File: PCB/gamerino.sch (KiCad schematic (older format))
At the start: 47 parts, among them J1 USB_B_Micro, J2 LT2, J3 RT2, P1 JOY1, P2 JOY2, P3 ICSP, P4 AUX, SW1 HATSWITCH, SW10 OPTS, SW11 X, SW12 B, SW13 A, SW14 Y, SW2 LT1, SW3 LT2, SW4 RT1, SW5 RT2, SW6 SEL, SW7 START, SW8 BACK, SW9 HOME, U1 MIC5219-3.3YM5, U2 ATmega32U4, U3 TCA9539, X1 16MHz

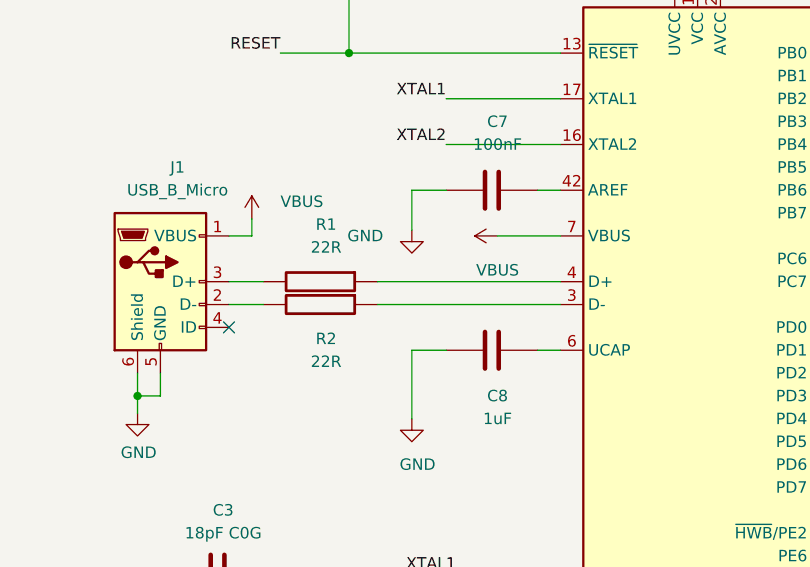
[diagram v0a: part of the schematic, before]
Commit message: Update Layout
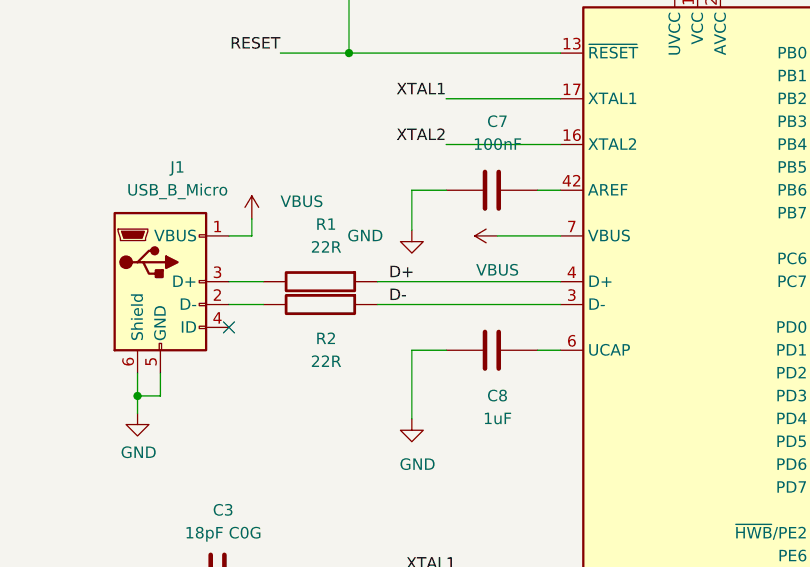
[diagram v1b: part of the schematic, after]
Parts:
- J2, J3: footprint gamerino:53398-0371 -> gamerino:Molex_PicoBlade_53047-0310_1x03_P1.25mm_Vertical
- R1, R2: footprint Resistor_SMD:R_0603_1608Metric -> Resistor_SMD:R_0402_1005Metric; MPN RT0603FRE0722RL -> (none); Manufacturer Yageo -> (none)
- SW10, SW6, SW7, SW8: footprint gamerino:TL1105-T -> gamerino:TL6210; MPN TL1105TF160Q -> TL6210AF200GQ
- SW9: footprint gamerino:TL1220 -> gamerino:TL3265; MPN TL1220R3BBBNN -> TL3265GQSCLR
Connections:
- net D-: now reaches R2.1, U2.3 (D-)
- net D+: now reaches R1.1, U2.4 (D+)
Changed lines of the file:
@@
 F 0 "R1" V 4175 4575 50  0000 C CNN
 F 1 "22R" V 4275 4575 50  0000 C CNN
-F 2 "Resistor_SMD:R_0603_1608Metric" V 4355 4550 30  0001 C CNN
+F 2 "Resistor_SMD:R_0402_1005Metric" V 4355 4550 30  0001 C CNN
 F 3 "" H 4425 4550 30  0000 C CNN
-F 4 "RT0603FRE0722RL" H 4425 4550 50  0001 C CNN "MPN"
-F 5 "Yageo" H 4425 4550 50  0001 C CNN "Manufacturer"
+F 4 "" H 4425 4550 50  0001 C CNN "MPN"
+F 5 "" H 4425 4550 50  0001 C CNN "Manufacturer"
 	1    4425 4550
 	0    1    1    0
@@
 F 0 "R2" V 4575 4675 50  0000 C CNN
 F 1 "22R" V 4675 4675 50  0000 C CNN
-F 2 "Resistor_SMD:R_0603_1608Metric" V 4355 4650 30  0001 C CNN
+F 2 "Resistor_SMD:R_0402_1005Metric" V 4355 4650 30  0001 C CNN
 F 3 "" H 4425 4650 30  0000 C CNN
-F 4 "RT0603FRE0722RL" H 4425 4650 50  0001 C CNN "MPN"
-F 5 "Yageo" H 4425 4650 50  0001 C CNN "Manufacturer"
+F 4 "" H 4425 4650 50  0001 C CNN "MPN"
+F 5 "" H 4425 4650 50  0001 C CNN "Manufacturer"
 	1    4425 4650
 	0    1    1    0
@@
 F 0 "J3" H 8050 9550 50  0000 C CNN
 F 1 "RT2" H 8050 9650 50  0000 C CNN
-F 2 "gamerino:53398-0371" H 8175 9925 50  0001 C CNN
+F 2 "gamerino:Molex_PicoBlade_53047-0310_1x03_P1.25mm_Vertical" H 8175 9925 50  0001 C CNN
 F 3 "" H 8175 9925 50  0001 C CNN
 F 4 "53047-0310" H 8175 9925 50  0001 C CNN "MPN"
@@
 F 0 "J2" H 8042 7739 50  0000 C CNN
 F 1 "LT2" H 8042 7830 50  0000 C CNN
-F 2 "gamerino:53398-0371" H 8175 8075 50  0001 C CNN
+F 2 "gamerino:Molex_PicoBlade_53047-0310_1x03_P1.25mm_Vertical" H 8175 8075 50  0001 C CNN
 F 3 "" H 8175 8075 50  0001 C CNN
 F 4 "53047-0310" H 8175 8075 50  0001 C CNN "MPN"
@@
 F 0 "SW9" H 14467 3431 50  0000 C CNN
 F 1 "HOME" H 14467 3340 50  0000 C CNN
-F 2 "gamerino:TL1220" H 14450 3250 50  0001 C CNN
+F 2 "gamerino:TL3265" H 14450 3250 50  0001 C CNN
 F 3 "" H 14450 3250 50  0001 C CNN
-F 4 "TL1220R3BBBNN" H 14450 3100 50  0001 C CNN "MPN"
+F 4 "TL3265GQSCLR" H 14450 3100 50  0001 C CNN "MPN"
 F 5 "E-Switch" H 14450 3100 50  0001 C CNN "Manufacturer"
 	1    14450 3100
@@
 F 0 "SW9" V 8846 8222 50  0000 R CNN
 F 1 "HOME" V 8755 8222 50  0000 R CNN
-F 2 "gamerino:TL1220" H 8800 8850 50  0001 C CNN
+F 2 "gamerino:TL3265" H 8800 8850 50  0001 C CNN
 F 3 "" H 8800 8850 50  0001 C CNN
-F 4 "TL1220R3BBBNN" H 8800 8700 50  0001 C CNN "MPN"
+F 4 "TL3265GQSCLR" H 8800 8700 50  0001 C CNN "MPN"
 F 5 "E-Switch" H 8800 8700 50  0001 C CNN "Manufacturer"
 	2    8800 8700
@@
 F 0 "SW6" H 14467 1781 50  0000 C CNN
 F 1 "SEL" H 14467 1690 50  0000 C CNN
-F 2 "gamerino:TL1105-T" H 14450 1100 50  0001 C CNN
+F 2 "gamerino:TL6210" H 14450 1100 50  0001 C CNN
 F 3 "" H 14450 1100 50  0001 C CNN
-F 4 "TL1105TF160Q" H 14450 1450 50  0001 C CNN "MPN"
+F 4 "TL6210AF200GQ" H 14450 1450 50  0001 C CNN "MPN"
 F 5 "E-Switch" H 14450 1450 50  0001 C CNN "Manufacturer"
 	1    14450 1450
@@
 F 0 "SW7" H 14467 2306 50  0000 C CNN
 F 1 "START" H 14467 2215 50  0000 C CNN
-F 2 "gamerino:TL1105-T" H 14450 1625 50  0001 C CNN
+F 2 "gamerino:TL6210" H 14450 1625 50  0001 C CNN
 F 3 "" H 14450 1625 50  0001 C CNN
-F 4 "TL1105TF160Q" H 14450 1975 50  0001 C CNN "MPN"
+F 4 "TL6210AF200GQ" H 14450 1975 50  0001 C CNN "MPN"
 F 5 "E-Switch" H 14450 1975 50  0001 C CNN "Manufacturer"
 	1    14450 1975
@@
 F 0 "SW8" H 14467 2856 50  0000 C CNN
 F 1 "BACK" H 14467 2765 50  0000 C CNN
-F 2 "gamerino:TL1105-T" H 14450 2175 50  0001 C CNN
+F 2 "gamerino:TL6210" H 14450 2175 50  0001 C CNN
 F 3 "" H 14450 2175 50  0001 C CNN
-F 4 "TL1105TF160Q" H 14450 2525 50  0001 C CNN "MPN"
+F 4 "TL6210AF200GQ" H 14450 2525 50  0001 C CNN "MPN"
 F 5 "E-Switch" H 14450 2525 50  0001 C CNN "Manufacturer"
 	1    14450 2525
@@
 F 0 "SW10" H 14467 3981 50  0000 C CNN
 F 1 "OPTS" H 14467 3890 50  0000 C CNN
-F 2 "gamerino:TL1105-T" H 14450 3800 50  0001 C CNN
+F 2 "gamerino:TL6210" H 14450 3800 50  0001 C CNN
 F 3 "" H 14450 3800 50  0001 C CNN
-F 4 "TL1105TF160Q" H 14450 3650 50  0001 C CNN "MPN"
+F 4 "TL6210AF200GQ" H 14450 3650 50  0001 C CNN "MPN"
 F 5 "E-Switch" H 14450 3650 50  0001 C CNN "Manufacturer"
 	1    14450 3650
@@
 LHOME
 NoConn ~ 5675 8575
+Text Label 4725 4550 0    50   ~ 0
+D+
+Text Label 4725 4650 0    50   ~ 0
+D-
 $EndSCHEMATC

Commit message: Update BOM
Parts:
- C10, C6, C7: MPN (none) -> 885012206020; Manufacturer (none) -> Wurth
- C3, C4: MPN (none) -> CGA2B2C0G1H180J050BA; Manufacturer (none) -> TDK
- C5, C8, C9: MPN (none) -> CGA3E1X7R1C105K080AC; Manufacturer (none) -> TDK
- P3: MPN (none) -> MTLW-103-07-G-S-230; Manufacturer (none) -> Samtec
- P4: MPN (none) -> CLM-108-02-F-D; Manufacturer (none) -> Samtec
- R1, R2: MPN (none) -> CRCW040222R0FKED; Manufacturer (none) -> Vishay
- R3, R5, R7: MPN (none) -> RC0603FR-0710KL; Manufacturer (none) -> Yageo
- R4: MPN (none) -> CRG0603F1K0; Manufacturer (none) -> TE
- R6, R8, R9: MPN (none) -> MCR03EZPFX2201; Manufacturer (none) -> ROHM
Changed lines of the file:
@@
 F 2 "Resistor_SMD:R_0603_1608Metric" V 8655 3550 30  0001 C CNN
 F 3 "" H 8725 3550 30  0000 C CNN
+F 4 "RC0603FR-0710KL" H 8725 3550 50  0001 C CNN "MPN"
+F 5 "Yageo" H 8725 3550 50  0001 C CNN "Manufacturer"
 	1    8725 3550
 	0    1    1    0
@@
 F 2 "Capacitor_SMD:C_0402_1005Metric" H 4013 6275 30  0001 C CNN
 F 3 "" H 3975 6425 60  0000 C CNN
+F 4 "CGA2B2C0G1H180J050BA" H 3975 6425 50  0001 C CNN "MPN"
+F 5 "TDK" H 3975 6425 50  0001 C CNN "Manufacturer"
 	1    3975 6425
 	0    1    1    0
@@
 F 2 "Capacitor_SMD:C_0402_1005Metric" H 4013 5675 30  0001 C CNN
 F 3 "" H 3975 5825 60  0000 C CNN
+F 4 "CGA2B2C0G1H180J050BA" H 3975 5825 50  0001 C CNN "MPN"
+F 5 "TDK" H 3975 5825 50  0001 C CNN "Manufacturer"
 	1    3975 5825
 	0    1    1    0
@@
 F 2 "Connector_PinHeader_2.54mm:PinHeader_2x03_P2.54mm_Vertical" H 4225 9975 50  0001 C CNN
 F 3 "" H 4225 9975 50  0001 C CNN
+F 4 "MTLW-103-07-G-S-230" H 4225 9975 50  0001 C CNN "MPN"
+F 5 "Samtec" H 4225 9975 50  0001 C CNN "Manufacturer"
 	1    4225 9975
 	-1   0    0    -1
@@
 F 2 "Capacitor_SMD:C_0603_1608Metric" H 10263 2950 30  0001 C CNN
 F 3 "" H 10225 3100 60  0000 C CNN
+F 4 "885012206020" H 10225 3100 50  0001 C CNN "MPN"
+F 5 "Wurth" H 10225 3100 50  0001 C CNN "Manufacturer"
 	1    10225 3100
 	0    1    1    0
@@
 F 2 "Capacitor_SMD:C_0603_1608Metric" H 5213 4700 30  0001 C CNN
 F 3 "" H 5175 4850 60  0000 C CNN
+F 4 "CGA3E1X7R1C105K080AC" H 5175 4850 50  0001 C CNN "MPN"
+F 5 "TDK" H 5175 4850 50  0001 C CNN "Manufacturer"
 	1    5175 4850
 	0    -1   -1   0
@@
 F 2 "Capacitor_SMD:C_0603_1608Metric" H 5213 4000 30  0001 C CNN
 F 3 "" H 5175 4150 60  0000 C CNN
+F 4 "885012206020" H 5175 4150 50  0001 C CNN "MPN"
+F 5 "Wurth" H 5175 4150 50  0001 C CNN "Manufacturer"
 	1    5175 4150
 	0    -1   -1   0
@@
 F 2 "Capacitor_SMD:C_0603_1608Metric" H 4088 1750 30  0001 C CNN
 F 3 "" H 4050 1900 60  0000 C CNN
+F 4 "CGA3E1X7R1C105K080AC" H 4050 1900 50  0001 C CNN "MPN"
+F 5 "TDK" H 4050 1900 50  0001 C CNN "Manufacturer"
 	1    4050 1900
 	-1   0    0    -1
@@
 F 2 "Resistor_SMD:R_0603_1608Metric" V 8430 4625 30  0001 C CNN
 F 3 "" H 8500 4625 30  0000 C CNN
+F 4 "MCR03EZPFX2201" H 8500 4625 50  0001 C CNN "MPN"
+F 5 "ROHM" H 8500 4625 50  0001 C CNN "Manufacturer"
 	1    8500 4625
 	1    0    0    -1
@@
 F 2 "Resistor_SMD:R_0603_1608Metric" V 8655 4625 30  0001 C CNN
 F 3 "" H 8725 4625 30  0000 C CNN
+F 4 "MCR03EZPFX2201" H 8725 4625 50  0001 C CNN "MPN"
+F 5 "ROHM" H 8725 4625 50  0001 C CNN "Manufacturer"
 	1    8725 4625
 	1    0    0    -1
@@
 F 2 "Resistor_SMD:R_0603_1608Metric" V 9155 3050 30  0001 C CNN
 F 3 "" H 9225 3050 30  0000 C CNN
+F 4 "MCR03EZPFX2201" H 9225 3050 50  0001 C CNN "MPN"
+F 5 "ROHM" H 9225 3050 50  0001 C CNN "Manufacturer"
 	1    9225 3050
 	1    0    0    -1
@@
 F 2 "Resistor_SMD:R_0402_1005Metric" V 4355 4550 30  0001 C CNN
 F 3 "" H 4425 4550 30  0000 C CNN
-F 4 "" H 4425 4550 50  0001 C CNN "MPN"
-F 5 "" H 4425 4550 50  0001 C CNN "Manufacturer"
+F 4 "CRCW040222R0FKED" H 4425 4550 50  0001 C CNN "MPN"
+F 5 "Vishay" H 4425 4550 50  0001 C CNN "Manufacturer"
 	1    4425 4550
 	0    1    1    0
@@
 F 2 "Resistor_SMD:R_0402_1005Metric" V 4355 4650 30  0001 C CNN
 F 3 "" H 4425 4650 30  0000 C CNN
-F 4 "" H 4425 4650 50  0001 C CNN "MPN"
-F 5 "" H 4425 4650 50  0001 C CNN "Manufacturer"
+F 4 "CRCW040222R0FKED" H 4425 4650 50  0001 C CNN "MPN"
+F 5 "Vishay" H 4425 4650 50  0001 C CNN "Manufacturer"
 	1    4425 4650
 	0    1    1    0
@@
 F 2 "Capacitor_SMD:C_0603_1608Metric" H 5513 2975 30  0001 C CNN
 F 3 "" H 5475 3125 60  0001 C CNN
+F 4 "CGA3E1X7R1C105K080AC" H 5475 3125 50  0001 C CNN "MPN"
+F 5 "TDK" H 5475 3125 50  0001 C CNN "Manufacturer"
 	1    5475 3125
 	0    1    1    0
@@
 F 2 "Capacitor_SMD:C_0603_1608Metric" H 4588 1750 30  0001 C CNN
 F 3 "" H 4550 1900 60  0000 C CNN
+F 4 "885012206020" H 4550 1900 50  0001 C CNN "MPN"
+F 5 "Wurth" H 4550 1900 50  0001 C CNN "Manufacturer"
 	1    4550 1900
 	-1   0    0    -1
@@
 F 2 "Resistor_SMD:R_0603_1608Metric" V 9030 8075 30  0001 C CNN
 F 3 "" H 9100 8075 30  0000 C CNN
+F 4 "CRG0603F1K0" H 9100 8075 50  0001 C CNN "MPN"
+F 5 "TE" H 9100 8075 50  0001 C CNN "Manufacturer"
 	1    9100 8075
 	1    0    0    -1
@@
 F 2 "Resistor_SMD:R_0603_1608Metric" V 4480 3050 30  0001 C CNN
 F 3 "" H 4550 3050 30  0000 C CNN
+F 4 "RC0603FR-0710KL" H 4550 3050 50  0001 C CNN "MPN"
+F 5 "Yageo" H 4550 3050 50  0001 C CNN "Manufacturer"
 	1    4550 3050
 	-1   0    0    1
@@
 F 2 "Connector_PinSocket_1.00mm:PinSocket_2x08_P1.00mm_Vertical_SMD" H 6075 8325 50  0001 C CNN
 F 3 "" H 6075 8325 50  0001 C CNN
+F 4 "CLM-108-02-F-D" H 6075 8325 50  0001 C CNN "MPN"
+F 5 "Samtec" H 6075 8325 50  0001 C CNN "Manufacturer"
 	1    6075 8325
 	-1   0    0    1
@@
 F 2 "Resistor_SMD:R_0603_1608Metric" V 7275 5675 30  0001 C CNN
 F 3 "" H 7425 5650 30  0000 C CNN
+F 4 "RC0603FR-0710KL" H 7425 5650 50  0001 C CNN "MPN"
+F 5 "Yageo" H 7425 5650 50  0001 C CNN "Manufacturer"
 	1    7425 5650
 	0    1    1    0
